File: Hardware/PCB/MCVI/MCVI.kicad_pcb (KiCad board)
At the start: 2 copper layers, 125.5 x 111 mm, 60 parts, among them IC2 TL074, IC3 TL074, J1 Conn_01x02, J10 AudioJack2, J11 AudioJack2, J12 AudioJack2, J13 AudioJack2, J14 AudioJack2, J15 AudioJack2, J16 AudioJack2, J2 Synth_power_2x5, J3 Conn_01x06, J4 Conn_01x10, J8 Conn_01x10, J9 AudioJack2, U1 6N137

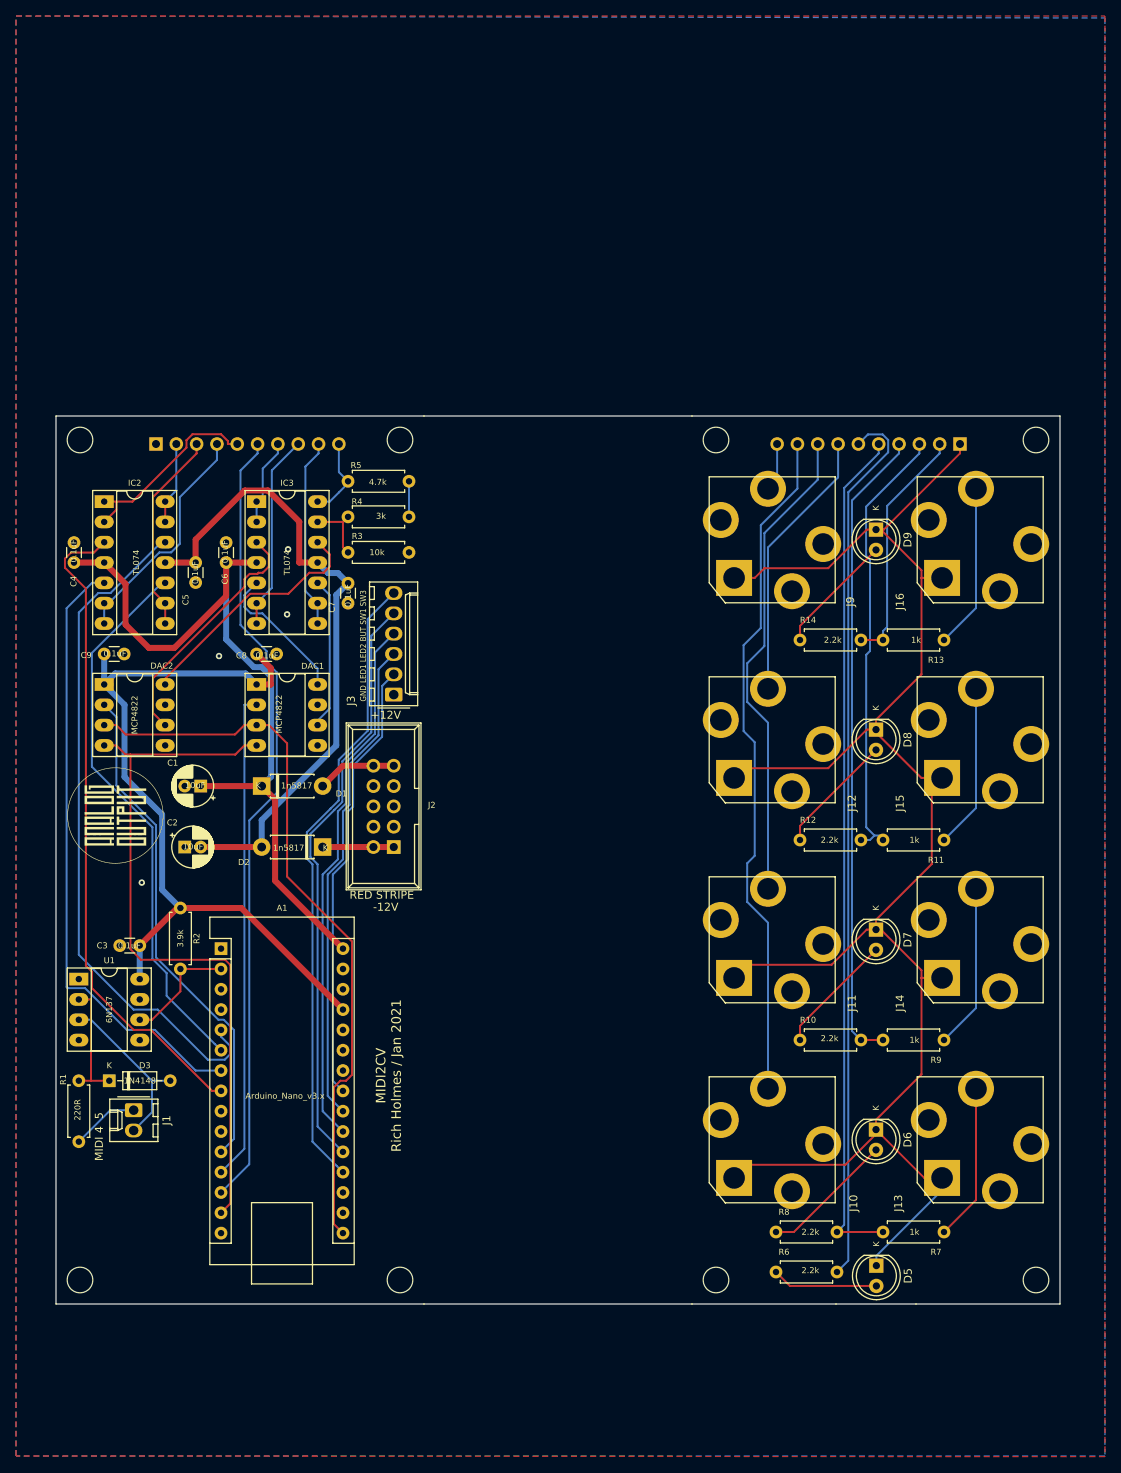
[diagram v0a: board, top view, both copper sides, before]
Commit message: New PCB layout
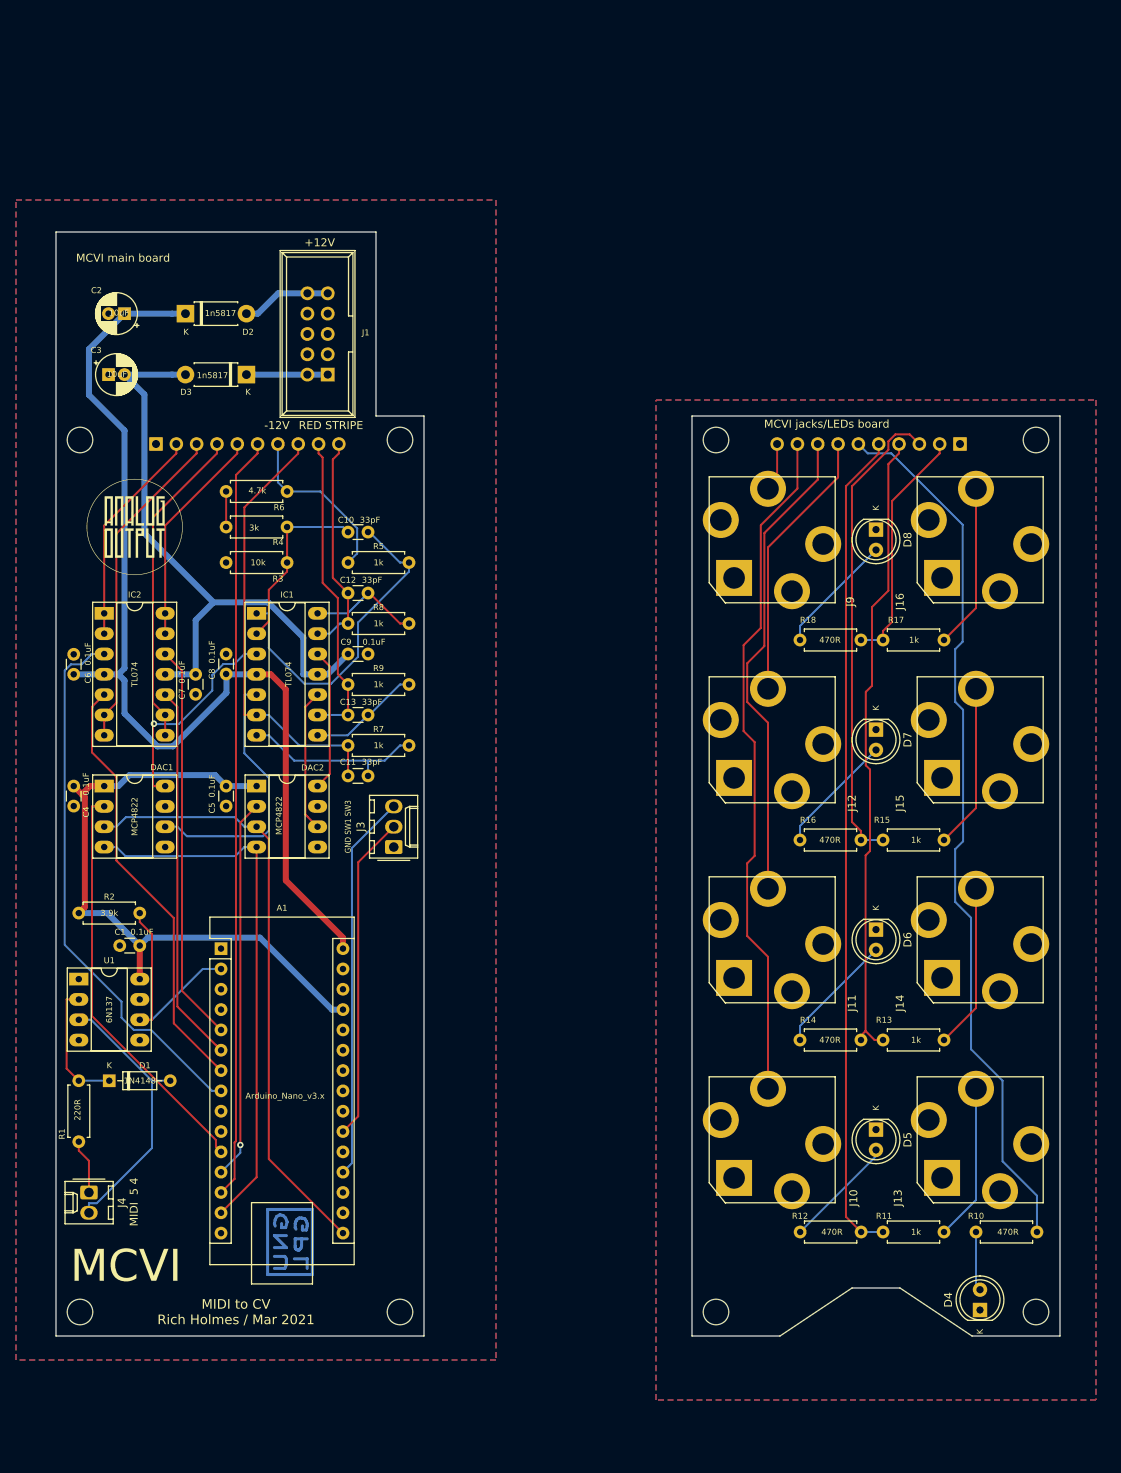
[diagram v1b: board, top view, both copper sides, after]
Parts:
- removed the C1 at (57.6, 110.3)
- removed the D1 at (65.2, 110.3)
- removed the J2 at (81.7, 117.9)
- added C10: 33pF, ao_tht:C_Disc_D3.0mm_W1.6mm_P2.50mm, F.Cu at (78.5, 78.5)
- added C11: 33pF, ao_tht:C_Disc_D3.0mm_W1.6mm_P2.50mm, F.Cu at (78.5, 109.0)
- added C12: 33pF, ao_tht:C_Disc_D3.0mm_W1.6mm_P2.50mm, F.Cu at (78.5, 86.1)
- added C13: 33pF, ao_tht:C_Disc_D3.0mm_W1.6mm_P2.50mm, F.Cu at (78.5, 101.4)
- added C3: 10uF, ao_tht:CP_Radial_D5.0mm_P2.00mm, F.Cu at (46.1, 58.8)
- added D3: 1n5817, ao_tht:D_DO-41_SOD81_P7.62mm_Horizontal, F.Cu at (63.3, 58.8)
- added J4: 2 pin Molex header, Connector_Molex:Molex_KK-254_AE-6410-02A_1x02_P2.54mm_Vertical, F.Cu at (43.6, 161.1)
- added R5: 1k, ao_tht:R_Axial_DIN0207_L6.3mm_D2.5mm_P7.62mm_Horizontal, F.Cu at (76.0, 82.3)
- added R7: 1k, ao_tht:R_Axial_DIN0207_L6.3mm_D2.5mm_P7.62mm_Horizontal, F.Cu at (76.0, 105.2)
- added R8: 1k, ao_tht:R_Axial_DIN0207_L6.3mm_D2.5mm_P7.62mm_Horizontal, F.Cu at (76.0, 89.9)
- added R9: 1k, ao_tht:R_Axial_DIN0207_L6.3mm_D2.5mm_P7.62mm_Horizontal, F.Cu at (76.0, 97.6)
- added REF**: Symbol_GNU-GPL_CopperTop_Small, Symbol:Symbol_GNU-GPL_CopperTop_Small, B.Cu at (69.0, 167.2)
- G***2: footprint midi2cv_ao:midi2cv_ao_panel_holes -> MCVI:MCVI_panel_holes
- J1: value Conn_01x02 -> Synth_power_2x5; footprint Connector_Molex:Molex_KK-254_AE-6410-02A_1x02_P2.54mm_Vertical -> ao_tht:Power_Header
- J2: renamed from J4; value Conn_01x10 -> 10 pin header
- J3: value Conn_01x06 -> 3 pin Molex header; footprint Connector_Molex:Molex_KK-254_AE-6410-06A_1x06_P2.54mm_Vertical -> Connector_Molex:Molex_KK-254_AE-6410-03A_1x03_P2.54mm_Vertical
- J8: value Conn_01x10 -> 10 pin socket
- R10: renamed from R6; value 2.2k -> 470R
- R12: renamed from R8; value 2.2k -> 470R
- R14: renamed from R10; value 2.2k -> 470R
- R16: renamed from R12; value 2.2k -> 470R
- R18: renamed from R14; value 2.2k -> 470R
- moved J1 95.1 mm to (73.5, 58.8), turned to 180 degrees
- moved D2 68.8 mm to (55.7, 51.2), turned to 0 degrees
- moved C2 67.1 mm to (48.1, 51.2), turned to 180 degrees
- moved G***1 36.1 mm to (49.3, 77.9), turned to 0 degrees
- moved R10 25.5 mm to (154.5, 166.0)
- moved IC1 23.6 mm to (64.6, 88.7)
- moved IC2 23.6 mm to (45.5, 88.7)
- moved R3 22.9 mm to (60.8, 82.3), turned to 0 degrees
- moved R4 22.9 mm to (60.8, 77.9), turned to 0 degrees
- moved J3 19.0 mm to (81.7, 117.9)
- moved C5 16.9 mm to (60.8, 110.3), turned to 270 degrees
- moved C4 16.9 mm to (41.7, 110.3), turned to 270 degrees
- moved D4 14.1 mm to (155.0, 175.8), turned to 90 degrees
- moved C6 14.0 mm to (41.7, 96.3)
- moved C7 14.0 mm to (57.0, 98.8)
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- renumbered C3 to C1, C9 to C4, C8 to C5, C4 to C6, C5 to C7, C6 to C8, C7 to C9, D3 to D1, D5 to D4, D6 to D5, D7 to D6, D8 to D7, D9 to D8, DAC2 to DAC1, DAC1 to DAC2, IC2 to IC1, IC3 to IC2, R7 to R11, R9 to R13, R11 to R15, R13 to R17, R5 to R6
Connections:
- net Net-(J8-Pad2) renamed /Panel components/CLOCK_4PQ_C
- net Net-(J8-Pad3) renamed /Panel components/CLOCK_1PQ_C
- net Net-(J8-Pad4) renamed /Panel components/TRIGGER_C
- net Net-(J8-Pad5) renamed /Panel components/GATE_C
- net Net-(J8-Pad6) renamed /Panel components/MIDI_LED_C
- A1 pad 20: /SW1 -> Net-(A1-Pad20)
- A1 pad 21: /BUT -> /SW1
- A1 pad 22: /PROG_LED1 -> Net-(A1-Pad22)
- A1 pad 23: /PROG_LED2 -> Net-(A1-Pad23)
- A1 pad 7: /CLOCK_B -> /CLOCK_1PQ_B
- A1 pad 8: /CLOCK_4_B -> /CLOCK_4PQ_B
- C2 pad 1: GND -> +12V
- C2 pad 2: -12V -> GND
- D2 pad 1: Net-(D2-Pad1) -> +12V
- D2 pad 2: -12V -> Net-(D2-Pad2)
- DAC1 pad 6: Net-(DAC2-Pad6) -> /VELOCITY_B
- DAC1 pad 8: Net-(DAC2-Pad8) -> /NOTE_B
- DAC2 pad 6: Net-(DAC1-Pad6) -> /CONTROL_B
- DAC2 pad 8: Net-(DAC1-Pad8) -> /PITCH_BEND_B
- IC1 pad 1: /CLOCK_4_A -> Net-(C10-Pad1)
- IC1 pad 10: /TRIGGER_B -> /CONTROL_B
- IC1 pad 12: /GATE_B -> /PITCH_BEND_B
- IC1 pad 13: /GATE_A -> /PITCH_BEND_A
- IC1 pad 14: /GATE_A -> Net-(C12-Pad1)
- IC1 pad 2: /CLOCK_4_A -> Net-(C10-Pad2)
- IC1 pad 3: /CLOCK_4_B -> /NOTE_B
- IC1 pad 5: /CLOCK_B -> /VELOCITY_B
- IC1 pad 6: /CLOCK_A -> /VELOCITY_A
- IC1 pad 7: /CLOCK_A -> Net-(C11-Pad1)
- IC1 pad 8: /TRIGGER_A -> Net-(C13-Pad1)
- IC1 pad 9: /TRIGGER_A -> /CONTROL_A
- IC2 pad 1: /VELOCITY_A -> /CLOCK_4PQ_A
- IC2 pad 10: Net-(DAC1-Pad6) -> /TRIGGER_B
- IC2 pad 12: Net-(DAC2-Pad8) -> /GATE_B
- IC2 pad 13: Net-(IC3-Pad13) -> /GATE_A
- IC2 pad 14: /NOTE_A -> /GATE_A
- IC2 pad 2: /VELOCITY_A -> /CLOCK_4PQ_A
- IC2 pad 3: Net-(DAC2-Pad6) -> /CLOCK_4PQ_B
- IC2 pad 5: Net-(DAC1-Pad8) -> /CLOCK_1PQ_B
- IC2 pad 6: /PITCH_BEND_A -> /CLOCK_1PQ_A
- IC2 pad 7: /PITCH_BEND_A -> /CLOCK_1PQ_A
- IC2 pad 8: /CONTROL_A -> /TRIGGER_A
- IC2 pad 9: /CONTROL_A -> /TRIGGER_A
- J1 pad 1: /MIDIPIN4 -> Net-(D3-Pad1)
- J1 pad 2: /MIDIPIN5 -> Net-(D3-Pad1)
- J11 pad T: /Panel components/PITCH_BEND -> /Panel components/VELOCITY
- J12 pad T: /Panel components/VELOCITY -> /Panel components/NOTE
- J13 pad T: /Panel components/CLOCK_4 -> /Panel components/GATE
- J14 pad T: /Panel components/CLOCK -> /Panel components/TRIGGER
- J15 pad T: /Panel components/TRIGGER -> /Panel components/CLOCK_1PQ
- J16 pad T: /Panel components/GATE -> /Panel components/CLOCK_4PQ
- J2 pad 10: /NOTE_A -> /PITCH_BEND_A
- J2 pad 2: /GATE_A -> /CLOCK_4PQ_A
- J2 pad 3: /TRIGGER_A -> /CLOCK_1PQ_A
- J2 pad 4: /CLOCK_A -> /TRIGGER_A
- J2 pad 5: /CLOCK_4_A -> /GATE_A
- J2 pad 7: /VELOCITY_A -> /NOTE_A
- J2 pad 8: /PITCH_BEND_A -> /VELOCITY_A
- J3 pad 2: /PROG_LED2 -> /SW1
- J3 pad 3: /PROG_LED1 -> /SW3
- J8 pad 10: /Panel components/NOTE -> /Panel components/PITCH_BEND
- J8 pad 7: /Panel components/VELOCITY -> /Panel components/NOTE
- J8 pad 8: /Panel components/PITCH_BEND -> /Panel components/VELOCITY
- J9 pad T: /Panel components/NOTE -> /Panel components/PITCH_BEND
- R11 pad 1: /Panel components/CLOCK_4 -> /Panel components/GATE
- R13 pad 1: /Panel components/CLOCK -> /Panel components/TRIGGER
- R15 pad 1: /Panel components/TRIGGER -> /Panel components/CLOCK_1PQ
- R17 pad 1: /Panel components/GATE -> /Panel components/CLOCK_4PQ
- R3 pad 2: Net-(IC3-Pad13) -> Net-(C10-Pad2)
- R4 pad 2: Net-(IC3-Pad13) -> Net-(C10-Pad2)
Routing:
- net GND1: track 220.2 -> 0.00 mm
- net /CLOCK_4_B: track 82.3 -> 0.00 mm
- net /CLOCK_B: track 77.0 -> 0.00 mm
- net /CLOCK_4PQ_B: track 0.00 -> 68.3 mm
- net /BUT: track 67.0 -> 0.00 mm
- net /PROG_LED1: track 61.4 -> 0.00 mm
- net /PROG_LED2: track 55.8 -> 0.00 mm
- net /CLOCK_1PQ_B: track 0.00 -> 54.3 mm
- net /Panel components/PITCH_BEND: track 60.3 -> 6.07 mm
- net /VELOCITY_A: track 11.6 -> 55.0 mm
- net /CLOCK_1PQ_A: track 0.00 -> 41.5 mm
- net Net-(C10-Pad1): track 0.00 -> 41.4 mm
- net /GATE_B: track 85.4 -> 49.9 mm
- net /VELOCITY_B: track 0.00 -> 33.5 mm
- net /SW1: track 73.3 -> 40.7 mm
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- added copper zone on B.Cu, net GND1
- added copper zone on F.Cu, net GND1
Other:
- board size 125.5 x 111 mm -> 125.5 x 138 mm
- board text added: "GND SW1 SW3"
- board text added: "Github repo https://github.com/holmesrichards/MCVI Based on design by Larry McGovern https://github.com/elkayem/midi2cv GPL3"
- board text added: "MCVI"
- board text added: "MCVI jacks/LEDs board"
- board text added: "MCVI main board"
- board text added: "MIDI 5 4"
- board text added: "MIDI to CV Rich Holmes / Mar 2021"
- board text removed: "GND LED1 LED2 BUT SW1 SW3"
- board text removed: "Github repo https://github.com/holmesrichards/midi2cv_ao Based on design by Larry McGovern https://github.com/elkayem/midi2cv"
- board text removed: "MIDI 4 5"
- board text removed: "MIDI2CV Rich Holmes / Jan 2021"
